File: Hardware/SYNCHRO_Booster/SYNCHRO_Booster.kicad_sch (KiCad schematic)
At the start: 41 parts, among them IC1 L6203, J1 Conn_01x02_Pin, J2 RJ45, U1 LM393P, U2 6N137, U3 6N137, U4 MAX485E, U5 MAX485E

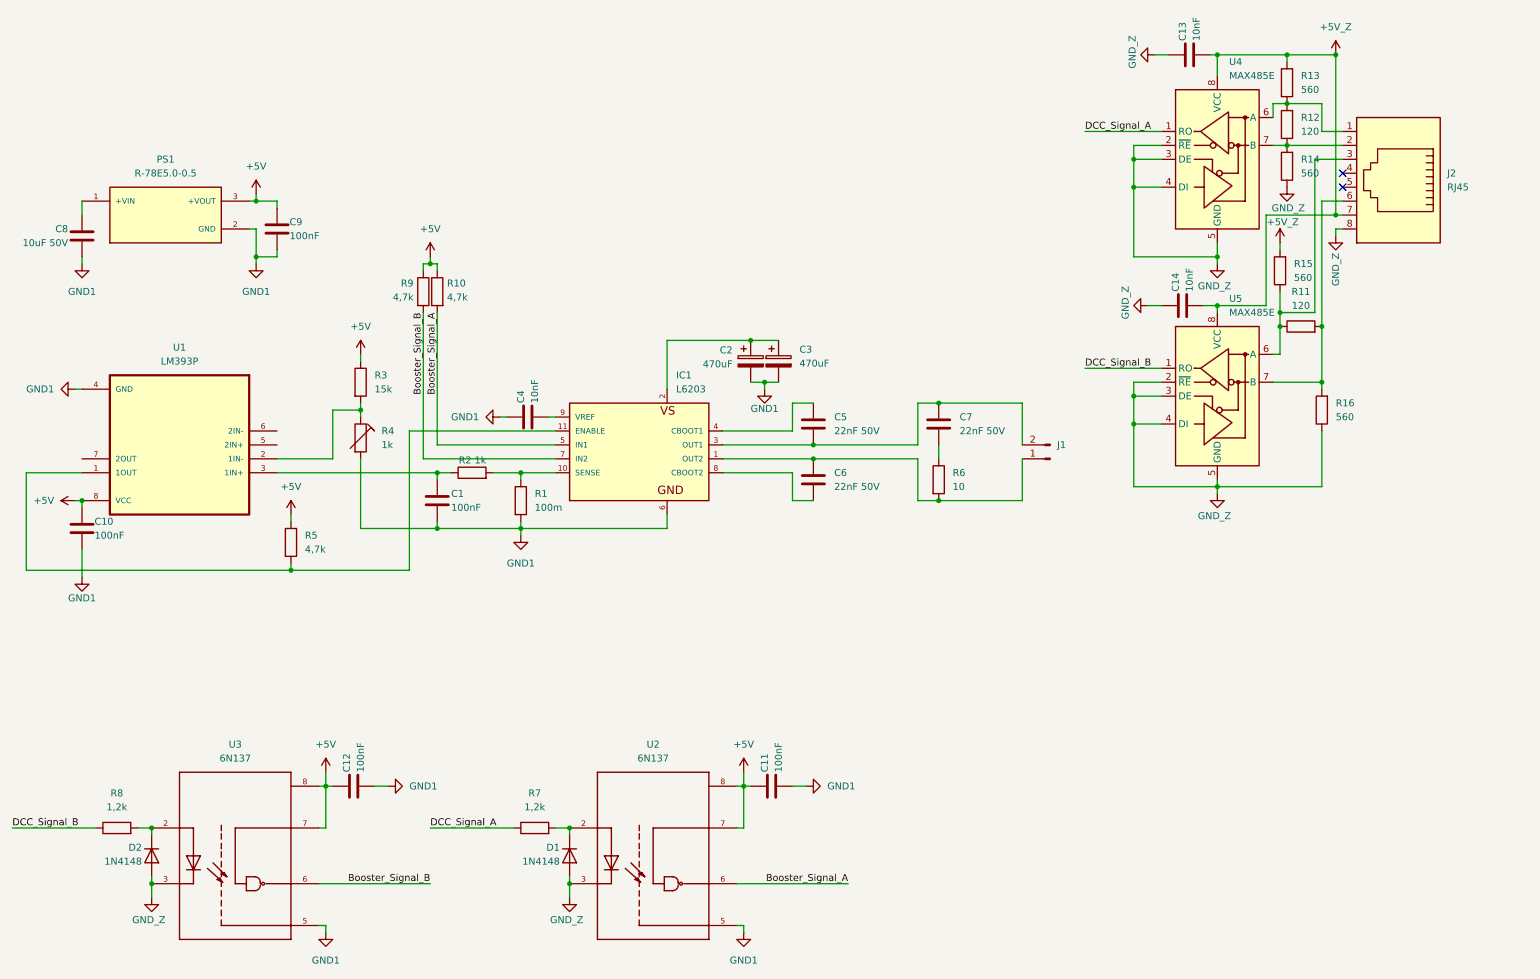
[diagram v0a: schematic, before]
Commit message: Booster Schematic Update
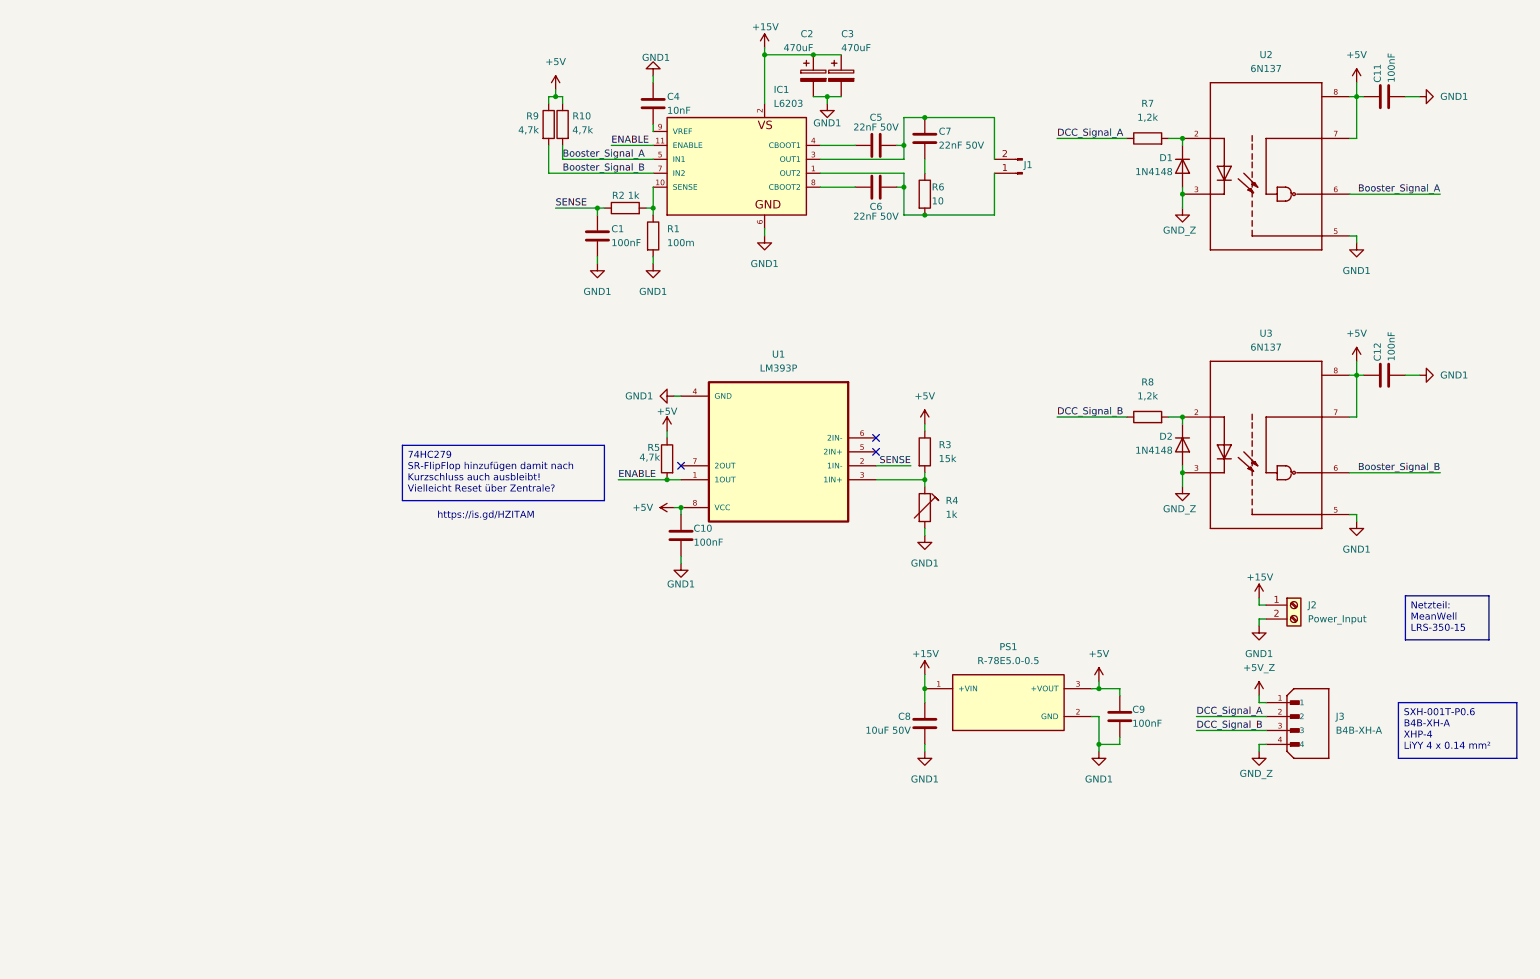
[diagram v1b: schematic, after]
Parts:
- removed C13, C14: 10nF, symbol Device:C
- removed J2: RJ45, symbol Connector:RJ45
- removed R11, R12: 120, symbol Device:R
- removed R13, R14, R15, R16: 560, symbol Device:R
- removed U4, U5: MAX485E, Package_SO:SOIC-8_3.9x4.9mm_P1.27mm, symbol Interface_UART:MAX485E
- added J2: Power_Input, TerminalBlock_Phoenix:TerminalBlock_Phoenix_MKDS-1,5-2-5.08_1x02_P5.08mm_Horizontal, symbol Connector:Screw_Terminal_01x02
- added J3: B4B-XH-A, symbol SYNCHRO_Library:B4B-XH-A_LF__SN_
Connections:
- net +5V_Z: now also J3.1
- net DCC_Signal_A: now also J3.2
- net DCC_Signal_B: now also J3.3
- net GND1: now also J2.2 (Pin_2)
- net GND_Z: now also J3.4
- net +15V: now reaches C8.1, PS1.1 (+VIN)
- net +15V: now also C2.1, C3.1, IC1.2, J2.1 (Pin_1)
- net ENABLE: now reaches IC1.11 (ENABLE), R5.2, U1.1 (1OUT)
- net SENSE: now reaches C1.1, R2.1
- net SENSE: now also U1.2 (1IN-); no longer U1.3 (1IN+)
- net at R3.2, R4.1: now also U1.3 (1IN+); no longer U1.2 (1IN-)
- no-connect marks 2 -> 3
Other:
- note added: "https://is.gd/HZITAM"
- moved on the sheet: C1, C10, C11, C12, C2, C3, C4, C5, C6, C7, C8, C9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
